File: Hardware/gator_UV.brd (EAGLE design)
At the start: 38.1 x 25.4 mm, 53 parts, among them J1 GATORGATOR_MINI, J2 GATORGATOR_MINI, J3 GATORGATOR_MINI, J4 GATORGATOR_MINI, J5 GATORGATOR_MINI, J6 GATORGATOR_MINI, J7 GATORGATOR_MINI, J8 GATORGATOR_MINI, Q1 2.5A/30V/105mΩ, U1 VEML6070"

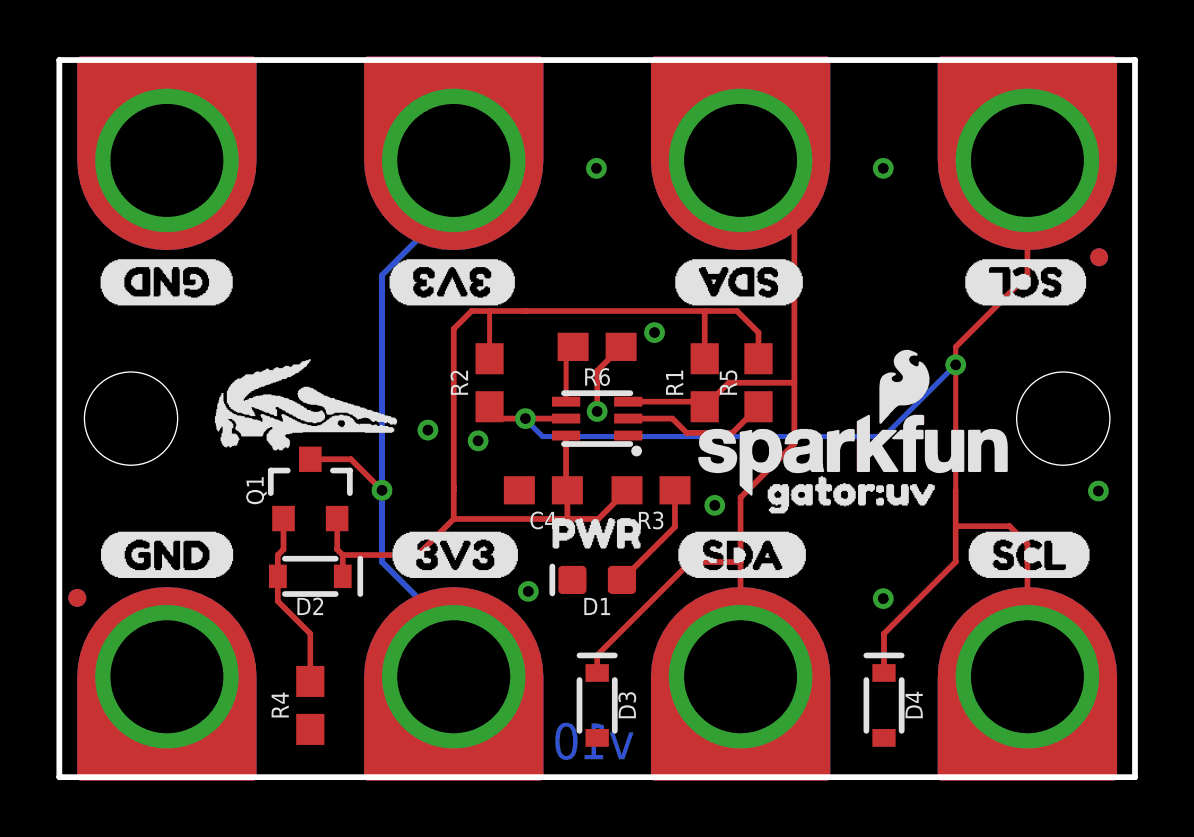
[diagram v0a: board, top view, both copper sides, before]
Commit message: qc double check changes
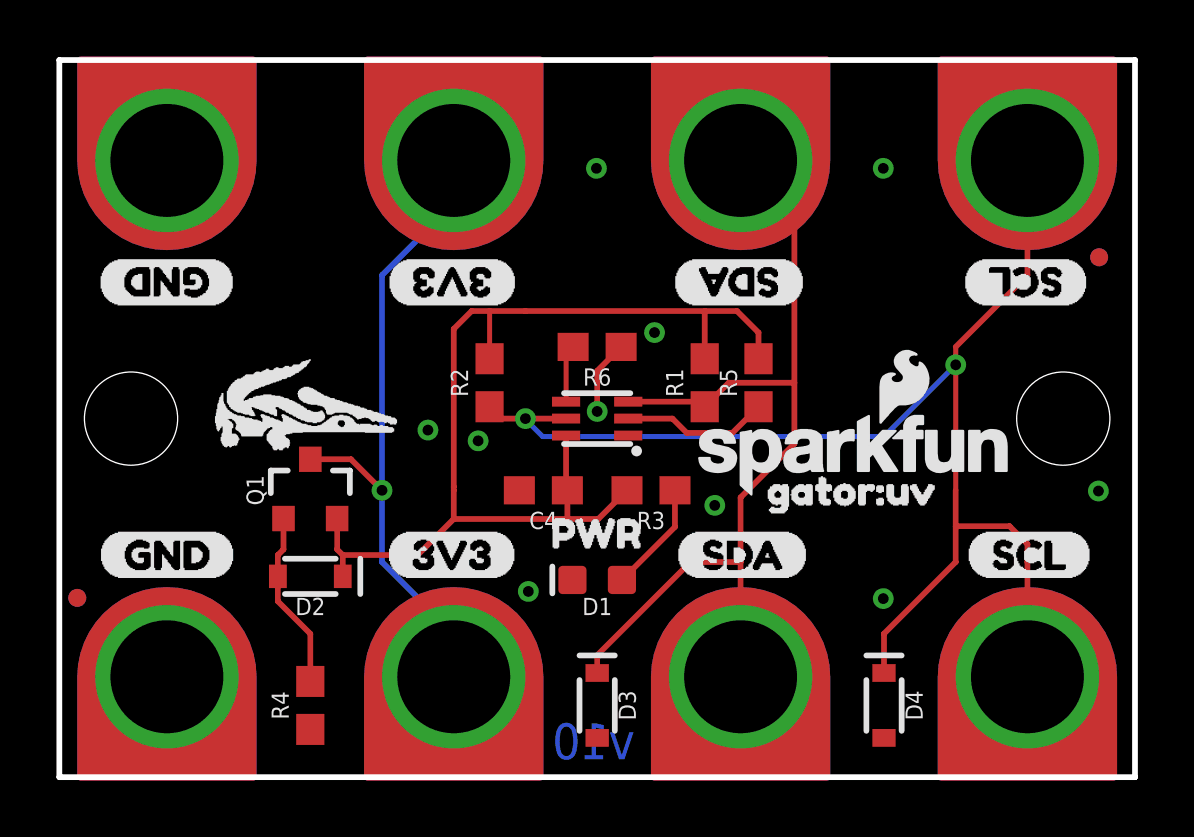
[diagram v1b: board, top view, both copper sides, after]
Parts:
- U1: value VEML6070" -> VEML6070
- moved U$11 0.13 mm to (32.0, 17.5)
- moved U$12 0.13 mm to (21.7, 17.5)
- moved U$21 0.13 mm to (36.6, 7.87)
- moved U$20 0.13 mm to (26.5, 7.87)
- moved U$3 0.13 mm to (11.6, 7.87)
- moved U$8 0.13 mm to (11.6, 17.5)
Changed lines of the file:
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@@
 <element name="J7" library="SparkFun-Connectors" package="GATOR_MINI" value="GATORGATOR_MINI" x="24.13" y="21.59" smashed="yes" rot="R180"/>
 <element name="J8" library="SparkFun-Connectors" package="GATOR_MINI" value="GATORGATOR_MINI" x="34.29" y="21.59" smashed="yes" rot="R180"/>
-<element name="U$3" library="buzzard_labels" package="3V33" value="" x="11.684" y="7.874" smashed="yes"/>
+<element name="U$3" library="buzzard_labels" package="3V33" value="" x="11.557" y="7.874" smashed="yes"/>
 <element name="U$4" library="buzzard_labels" package="GND0" value="" x="1.397" y="7.874" smashed="yes"/>
 <element name="U$5" library="buzzard_labels" package="SCL2" value="" x="32.131" y="7.874" smashed="yes"/>
 <element name="U$7" library="buzzard_labels" package="SDA1" value="" x="21.844" y="7.874" smashed="yes"/>
-<element name="U$8" library="buzzard_labels" package="3V33" value="" x="11.684" y="17.526" smashed="yes" rot="MR180"/>
+<element name="U$8" library="buzzard_labels" package="3V33" value="" x="11.557" y="17.526" smashed="yes" rot="MR180"/>
 <element name="U$9" library="buzzard_labels" package="GND0" value="" x="1.397" y="17.526" smashed="yes" rot="MR180"/>
-<element name="U$11" library="buzzard_labels" package="SCL2" value="" x="32.131" y="17.526" smashed="yes" rot="MR180"/>
-<element name="U$12" library="buzzard_labels" package="SDA1" value="" x="21.844" y="17.526" smashed="yes" rot="MR180"/>
+<element name="U$11" library="buzzard_labels" package="SCL2" value="" x="32.004" y="17.526" smashed="yes" rot="MR180"/>
+<element name="U$12" library="buzzard_labels" package="SDA1" value="" x="21.717" y="17.526" smashed="yes" rot="MR180"/>
 <element name="U$13" library="buzzard_labels" package="GND0" value="" x="6.223" y="17.526" smashed="yes" rot="R180"/>
 <element name="U$14" library="buzzard_labels" package="3V33" value="" x="16.256" y="17.526" smashed="yes" rot="R180"/>
@@
 <element name="U$18" library="buzzard_labels" package="GND0" value="" x="6.223" y="7.874" smashed="yes" rot="MR0"/>
 <element name="U$19" library="buzzard_labels" package="3V33" value="" x="16.256" y="7.874" smashed="yes" rot="MR0"/>
-<element name="U$20" library="buzzard_labels" package="SDA1" value="" x="26.416" y="7.874" smashed="yes" rot="MR0"/>
-<element name="U$21" library="buzzard_labels" package="SCL2" value="" x="36.449" y="7.874" smashed="yes" rot="MR0"/>
+<element name="U$20" library="buzzard_labels" package="SDA1" value="" x="26.543" y="7.874" smashed="yes" rot="MR0"/>
+<element name="U$21" library="buzzard_labels" package="SCL2" value="" x="36.576" y="7.874" smashed="yes" rot="MR0"/>
 <element name="D2" library="SparkFun-DiscreteSemi" package="SOD-323" value="3.6V" x="8.89" y="7.112" smashed="yes" rot="R180">
 <attribute name="NAME" x="8.89" y="6.35" size="0.6096" layer="25" font="vector" ratio="20" rot="R180" align="bottom-center"/>
@@
 </element>
 <element name="U$10" library="SparkFun-Aesthetics" package="ORDERING_INSTRUCTIONS" value="" x="1.27" y="-10.16"/>
-<element name="U1" library="SparkFun-Sensors" package="VEML6070" value="VEML6070&quot;" x="19.05" y="12.7" rot="R180"/>
+<element name="U1" library="SparkFun-Sensors" package="VEML6070" value="VEML6070" x="19.05" y="12.7" rot="R180">
+<attribute name="PROD_ID" value="SEN-14367" x="19.05" y="12.7" size="1.778" layer="27" rot="R180" display="off"/>
+<attribute name="VALUE" value="VEML6070" x="19.05" y="12.7" size="1.778" layer="27" rot="R180" display="off"/>
+</element>
 <element name="R5" library="SparkFun-Resistors" package="0603" value="10k" x="24.765" y="13.97" rot="R90">
 <attribute name="PROD_ID" value="RES-00824" x="24.765" y="13.97" size="1.778" layer="27" rot="R90" display="off"/>
